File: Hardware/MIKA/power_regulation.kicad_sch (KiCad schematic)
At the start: 11 parts, among them J1 Display_PWR, J2 Router_PWR

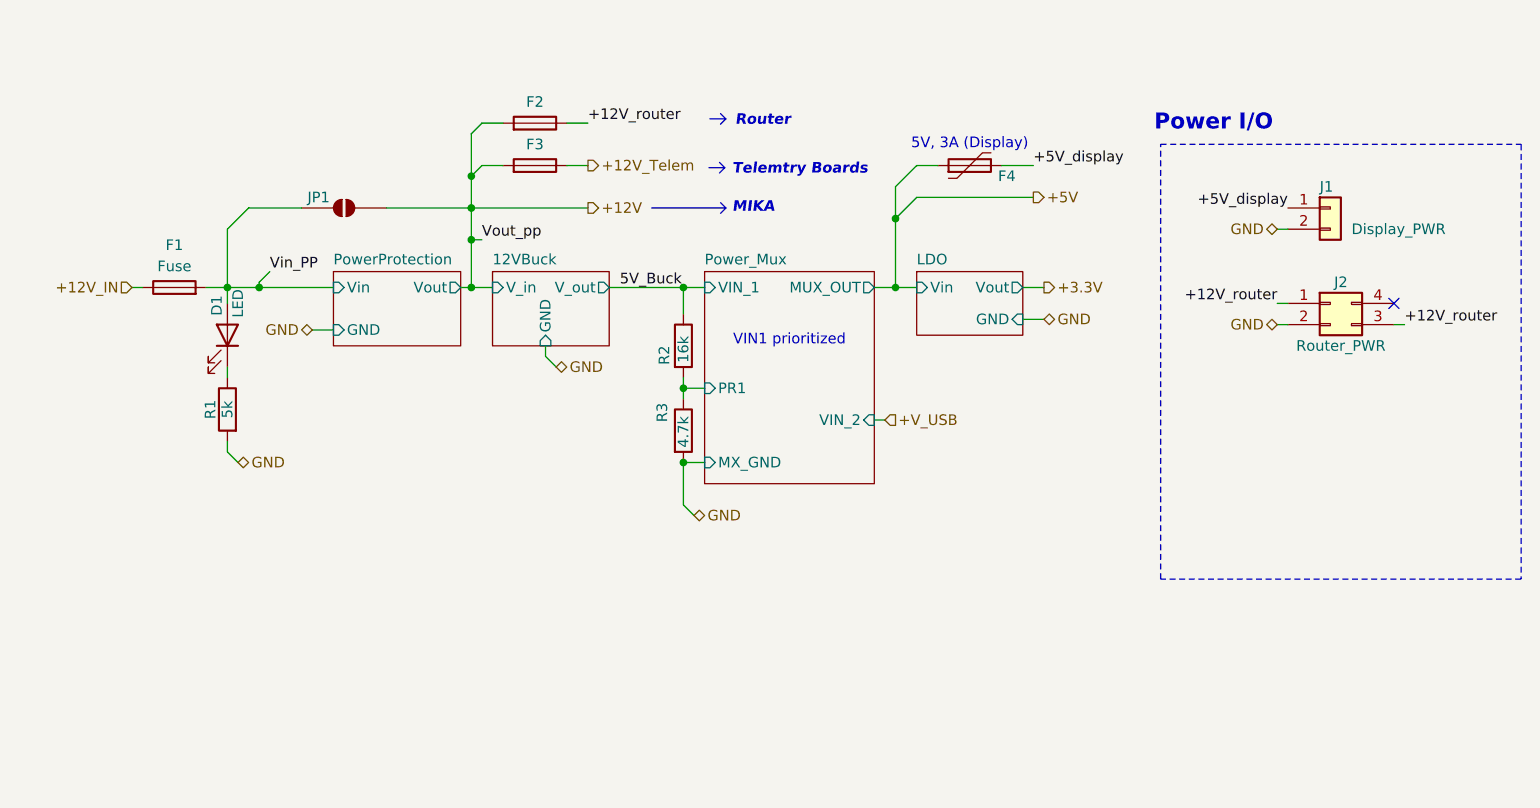
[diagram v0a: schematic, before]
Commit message: bahasdf;ladjsfhadf boooooooooooshksa
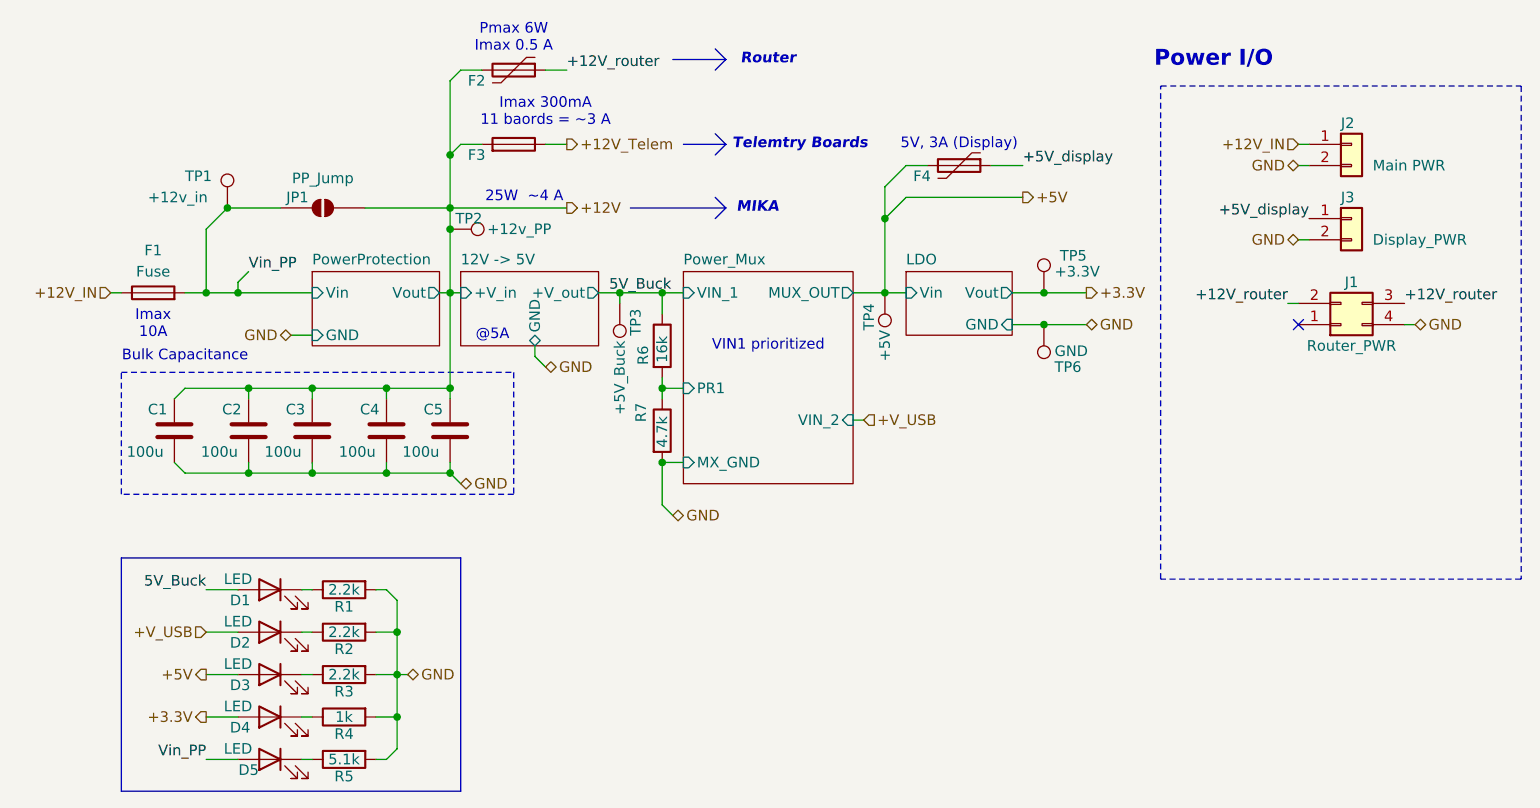
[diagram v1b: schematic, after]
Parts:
- removed F2: Fuse, LHRS_Power:Fuse-3557-2, symbol Device:Fuse
- added C1, C2, C3, C4, C5: 100u, symbol Device:C
- added D1, D2, D3, D4: LED, LED_SMD:LED_0603_1608Metric, symbol Device:LED
- added F2: Polyfuse, symbol Device:Polyfuse
- added J2: Main PWR, symbol Connector_Generic:Conn_01x02
- added R1, R2, R3: 2.2k, Resistor_SMD:R_0603_1608Metric_Pad0.98x0.95mm_HandSolder, symbol Device:R
- added R4: 1k, Resistor_SMD:R_0603_1608Metric_Pad0.98x0.95mm_HandSolder, symbol Device:R
- added TP1: +12v_in, symbol Connector:TestPoint
- added TP2: +12v_PP, symbol Connector:TestPoint
- added TP3: +5V_Buck, symbol Connector:TestPoint
- added TP4: +5V, symbol Connector:TestPoint
- added TP5: +3.3V, symbol Connector:TestPoint
- added TP6: GND, symbol Connector:TestPoint
- JP1: value SolderJumper_2_Open -> PP_Jump
- R5: renamed from R1; value 5k -> 5.1k
- renumbered D1 to D5, J2 to J1, J1 to J3, R2 to R6, R3 to R7
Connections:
- net +12V: now also C1.1, C2.1, C3.1, C4.1, C5.1, F2.2, TP2.1
- net +12V_IN: now also J2.1 (Pin_1)
- net +12V_router: now also J1.2 (Pin_2), F2.1; no longer J1.1 (Pin_1)
- net +3.3V: now also D4.2 (A), TP5.1
- net +5V: now also F4.2, D3.2 (A), TP4.1; no longer F4.1
- net +5V_display: now also F4.1; no longer F4.2
- net +V_USB: now also D2.2 (A)
- net 5V_Buck: now also D1.2 (A), TP3.1
- net GND: now also J1.4 (Pin_4), C1.2, C2.2, C3.2, C4.2, C5.2, J2.2 (Pin_2), R1.2, R2.2, R3.2, R4.2, TP6.1; no longer J1.2 (Pin_2)
- net Vin_PP: now also TP1.1
- new net: D1.1 (K), R1.1
- new net: D4.1 (K), R4.1
- new net: D2.1 (K), R2.1
- new net: D3.1 (K), R3.1
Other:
- removed sheet 12VBuck
- added sheet 12V -> 5V (12V_buck_5A.kicad_sch)
- note added: "25W ~4 A"
- note added: "@5A"
- note added: "Bulk Capacitance"
- note added: "Imax 10A"
- note added: "Imax 300mA 11 baords = ~3 A"
- note added: "Pmax 6W Imax 0.5 A"
- moved on the sheet: D5, F1, F3, J1, J3, JP1, R5, R6, R7
